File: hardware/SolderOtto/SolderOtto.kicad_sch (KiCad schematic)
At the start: 0 parts

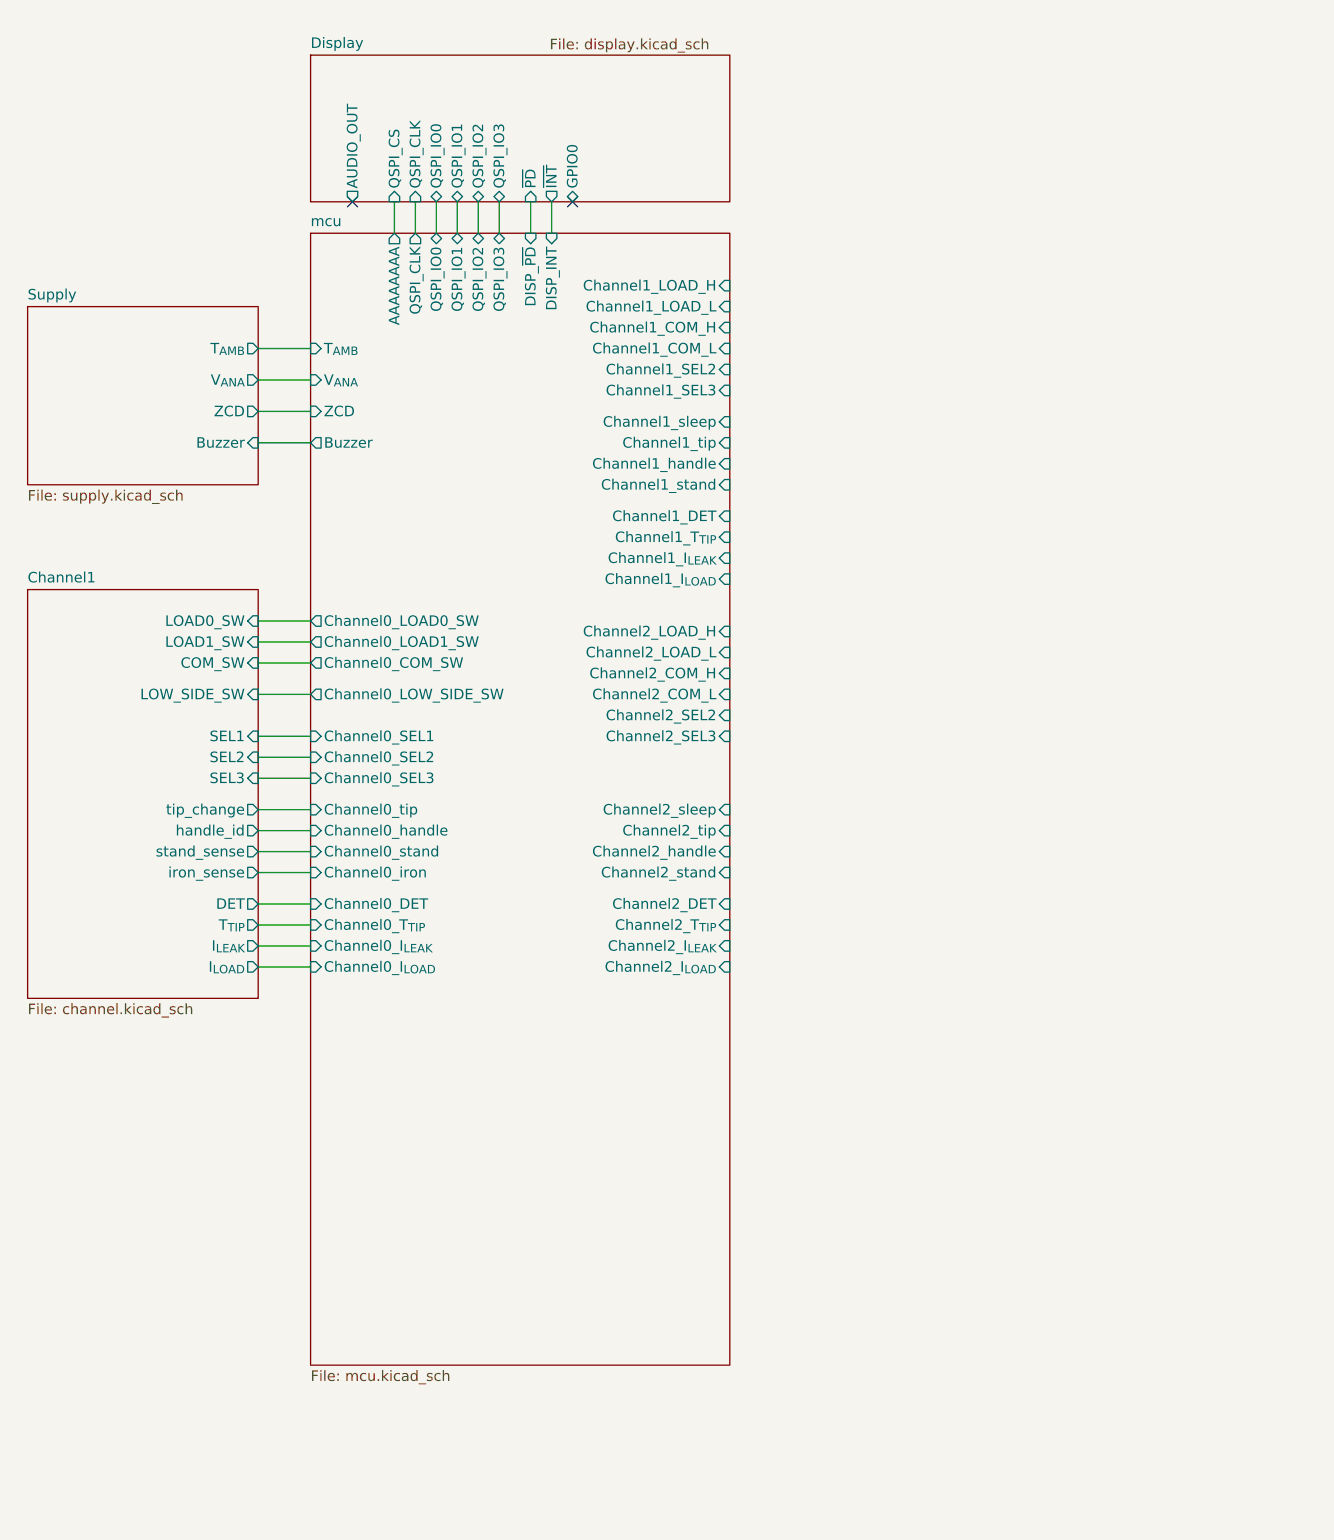
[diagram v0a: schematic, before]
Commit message: save wip
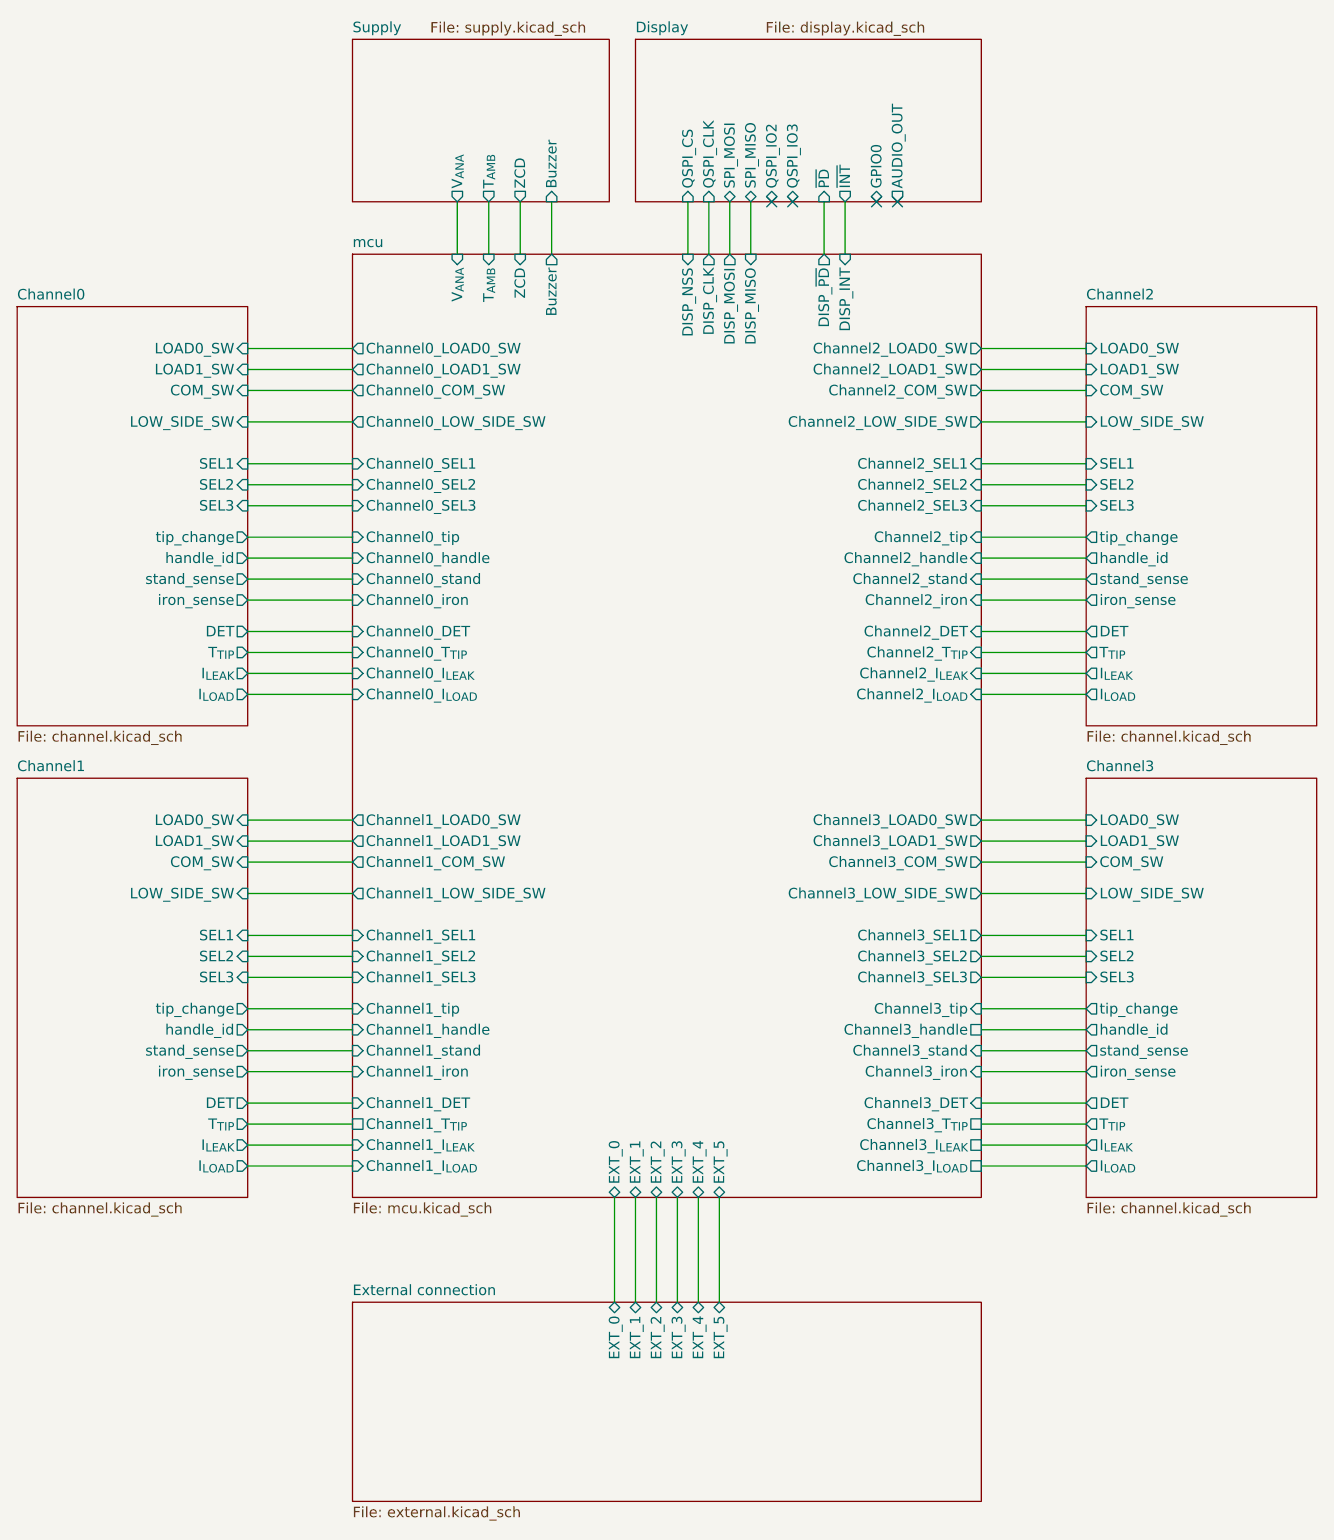
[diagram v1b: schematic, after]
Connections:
- no-connect marks 2 -> 4
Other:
- added sheet Channel0 (channel.kicad_sch)
- added sheet Channel2 (channel.kicad_sch)
- added sheet Channel3 (channel.kicad_sch)
- added sheet External connection (external.kicad_sch)
- sheet Display ports: added SPI_MISO, SPI_MOSI; removed QSPI_IO0, QSPI_IO1
- sheet mcu ports: added Channel1_COM_SW, Channel1_LOAD0_SW, Channel1_LOAD1_SW, Channel1_LOW_SIDE_SW, Channel1_SEL1, Channel1_iron, Channel2_COM_SW, Channel2_LOAD0_SW, Channel2_LOAD1_SW, Channel2_LOW_SIDE_SW, Channel2_SEL1, Channel2_iron, Channel3_COM_SW, Channel3_DET, Channel3_I_{LEAK}, Channel3_I_{LOAD}, Channel3_LOAD0_SW, Channel3_LOAD1_SW, Channel3_LOW_SIDE_SW, Channel3_SEL1, Channel3_SEL2, Channel3_SEL3, Channel3_T_{TIP}, Channel3_handle, Channel3_iron, Channel3_stand, Channel3_tip, DISP_CLK, DISP_MISO, DISP_MOSI, DISP_NSS, EXT_0, EXT_1, EXT_2, EXT_3, EXT_4, EXT_5; removed AAAAAAAA, Channel1_COM_H, Channel1_COM_L, Channel1_LOAD_H, Channel1_LOAD_L, Channel1_sleep, Channel2_COM_H, Channel2_COM_L, Channel2_LOAD_H, Channel2_LOAD_L, Channel2_sleep, QSPI_CLK, QSPI_IO0, QSPI_IO1, QSPI_IO2, QSPI_IO3
